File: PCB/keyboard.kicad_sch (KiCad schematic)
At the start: 139 parts, among them SW1 SW_Push, SW10 SW_Push, SW11 SW_Push, SW12 SW_Push, SW13 SW_Push, SW14 SW_Push, SW15 SW_Push, SW16 SW_Push, SW17 SW_Push, SW18 SW_Push, SW19 SW_Push, SW2 SW_Push, SW20 SW_Push, SW21 SW_Push, SW22 SW_Push, SW23 SW_Push, SW24 SW_Push, SW25 SW_Push, SW26 SW_Push, SW27 SW_Push, SW28 SW_Push, SW29 SW_Push, SW3 SW_Push, SW30 SW_Push, SW31 SW_Push, SW32 SW_Push, SW33 SW_Push, SW34 SW_Push, SW35 SW_Push, SW36 SW_Push, SW37 SW_Push, SW38 SW_Push, SW39 SW_Push, SW4 SW_Push, SW40 SW_Push, SW41 SW_Push, SW42 SW_Push, SW43 SW_Push, SW44 SW_Push, SW45 SW_Push, SW46 SW_Push, SW47 SW_Push, SW48 SW_Push, SW49 SW_Push, SW5 SW_Push, SW50 SW_Push, SW51 SW_Push, SW52 SW_Push, SW53 SW_Push, SW54 SW_Push, SW55 SW_Push, SW56 SW_Push, SW57 SW_Push, SW58 SW_Push, SW59 SW_Push, SW6 SW_Push, SW60 SW_Push, SW61 SW_Push, SW62 RotaryEncoder_Switch, SW63 RotaryEncoder_Switch, SW7 SW_Push, SW8 SW_Push, SW9 SW_Push, U1 Pico

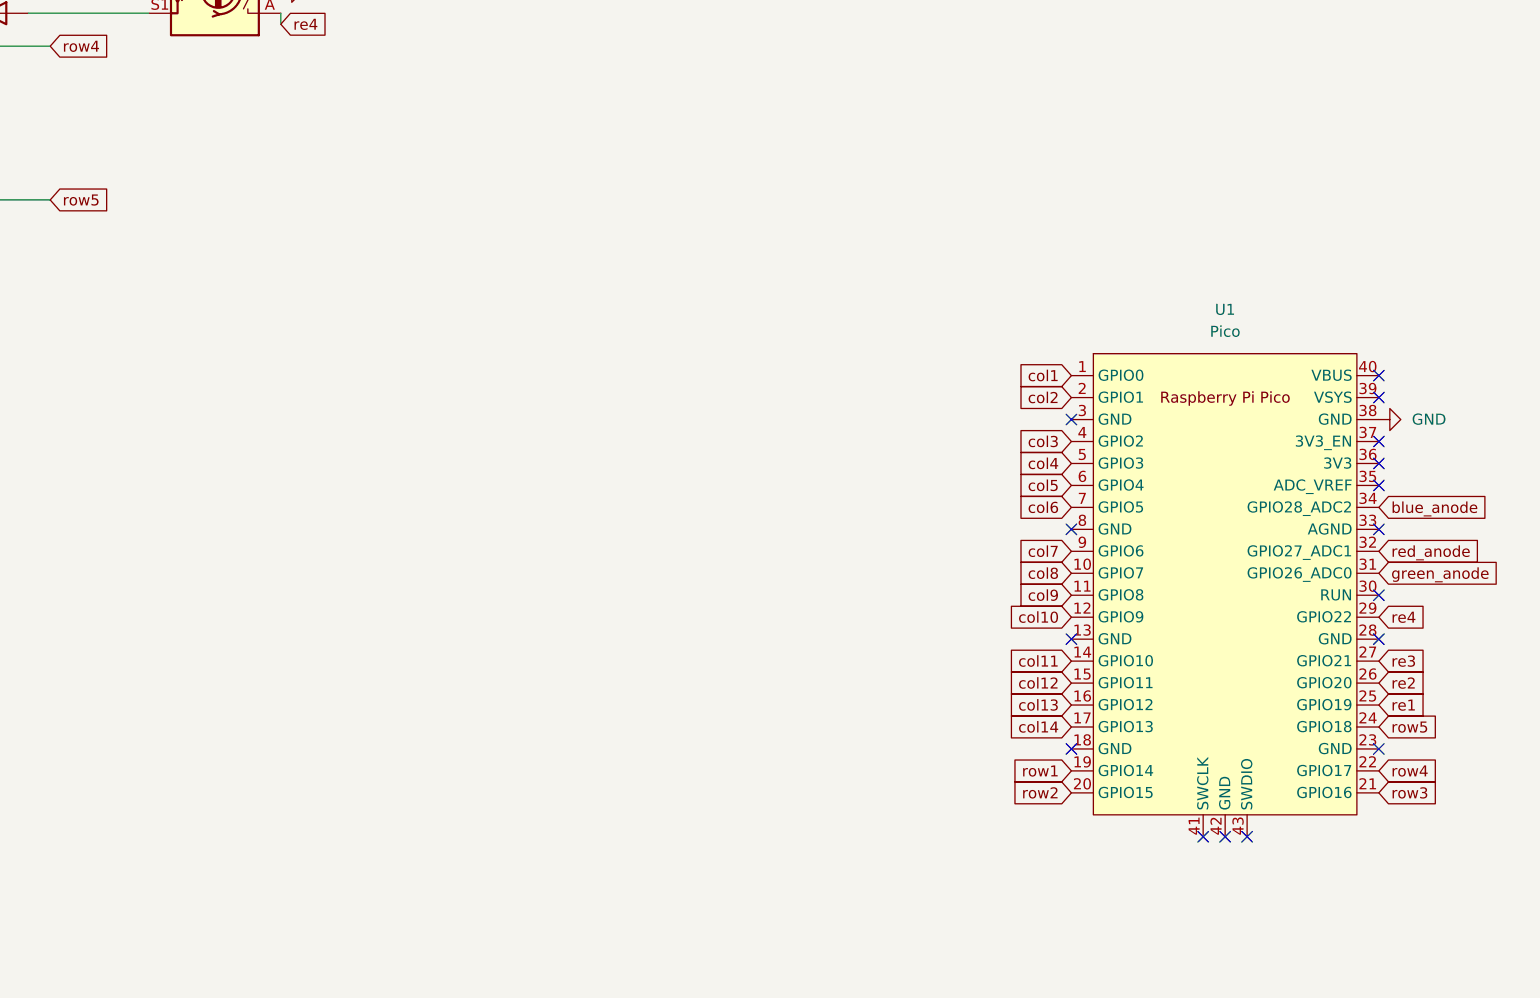
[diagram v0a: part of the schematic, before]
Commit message: Added PCB
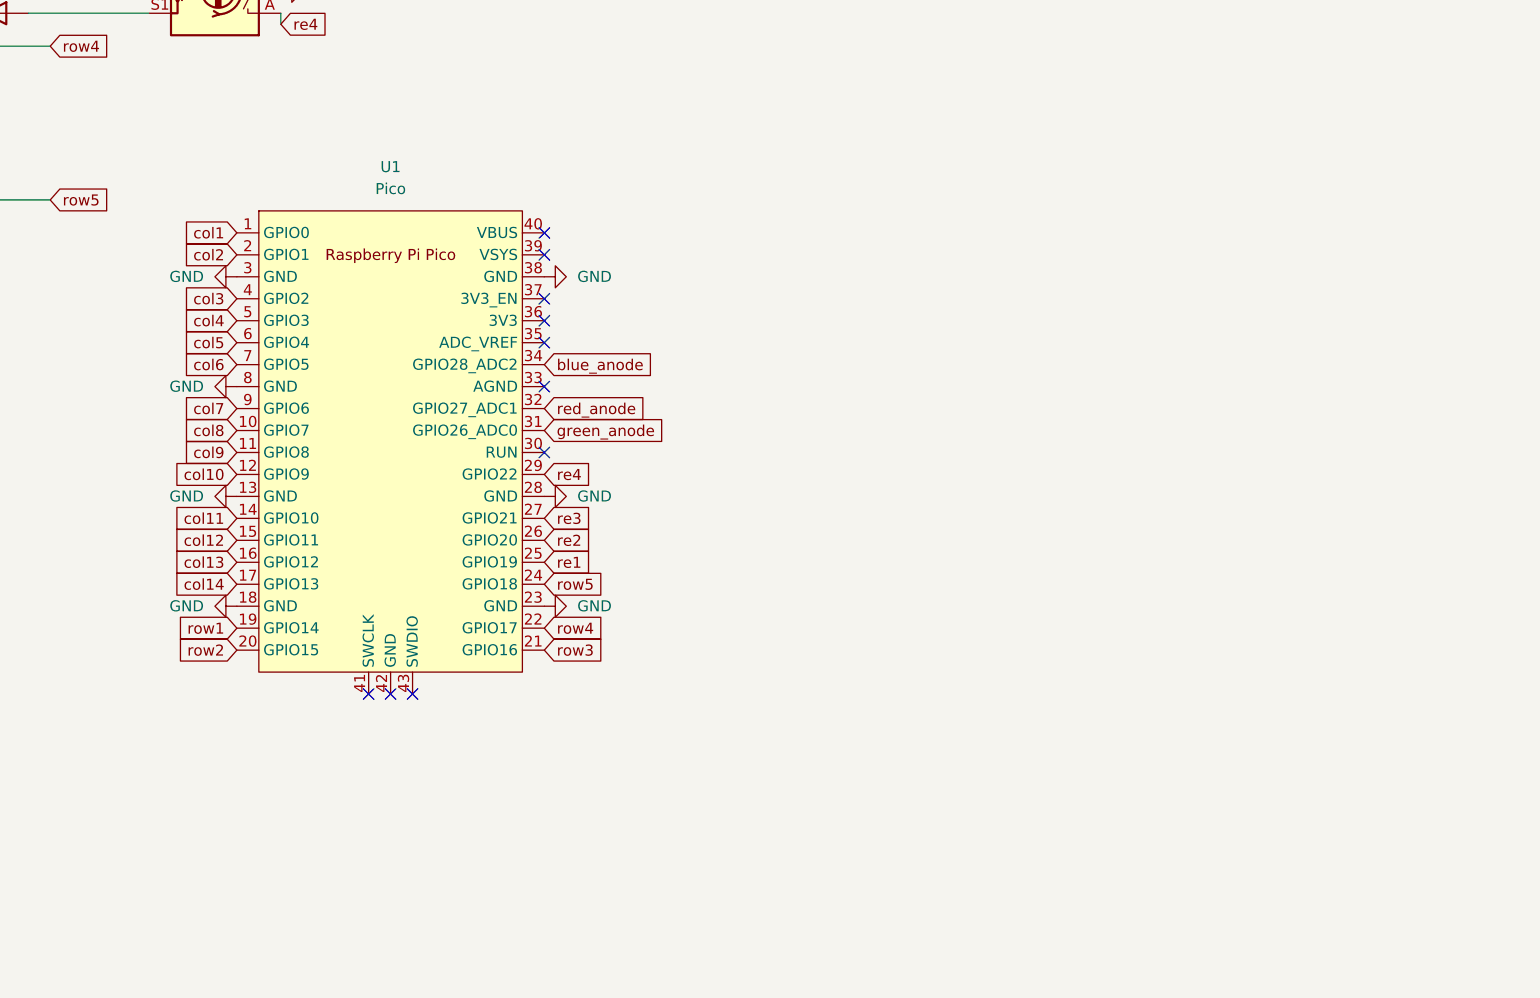
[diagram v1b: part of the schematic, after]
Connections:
- net GND: now also U1.13 (GND), U1.18 (GND), U1.23 (GND), U1.28 (GND), U1.3 (GND), U1.8 (GND)
- no-connect marks 16 -> 10
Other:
- moved on the sheet: U1
